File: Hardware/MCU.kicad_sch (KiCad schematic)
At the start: 37 parts, among them J5 Conn_01x05_Pin, Q1 BC847, SW1 SW_Push, SW2 SW_SPDT, U1 STM32F405RGT6, Y2 25MHz

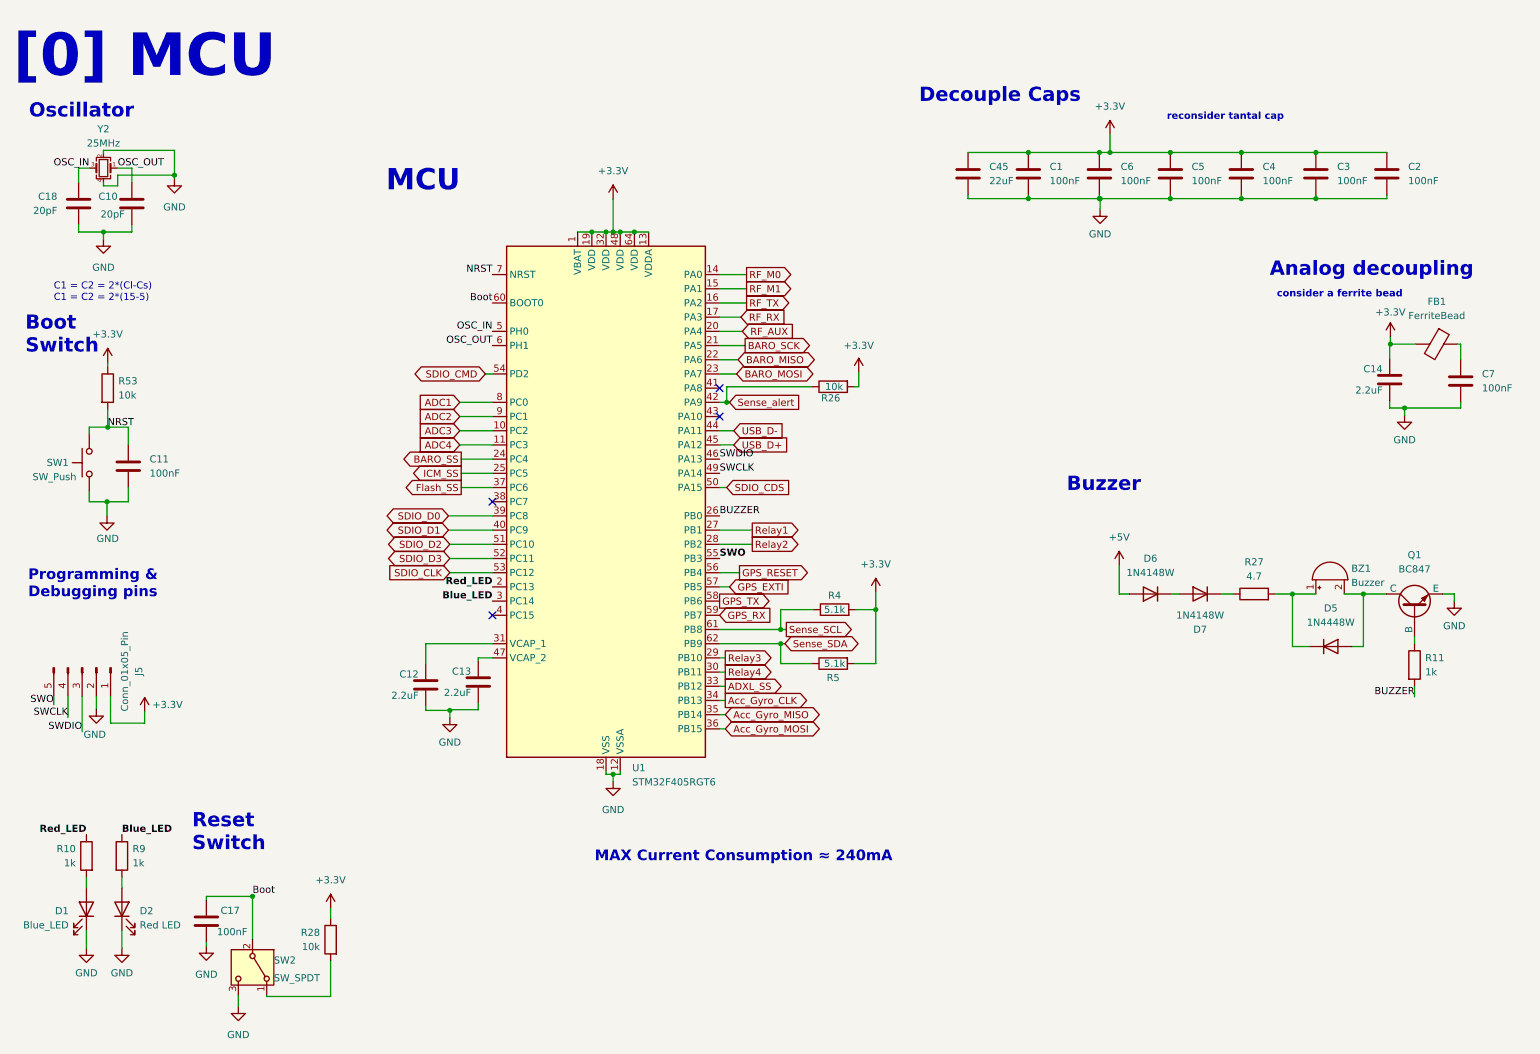
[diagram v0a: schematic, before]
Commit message: Changed footprints, generated BOM
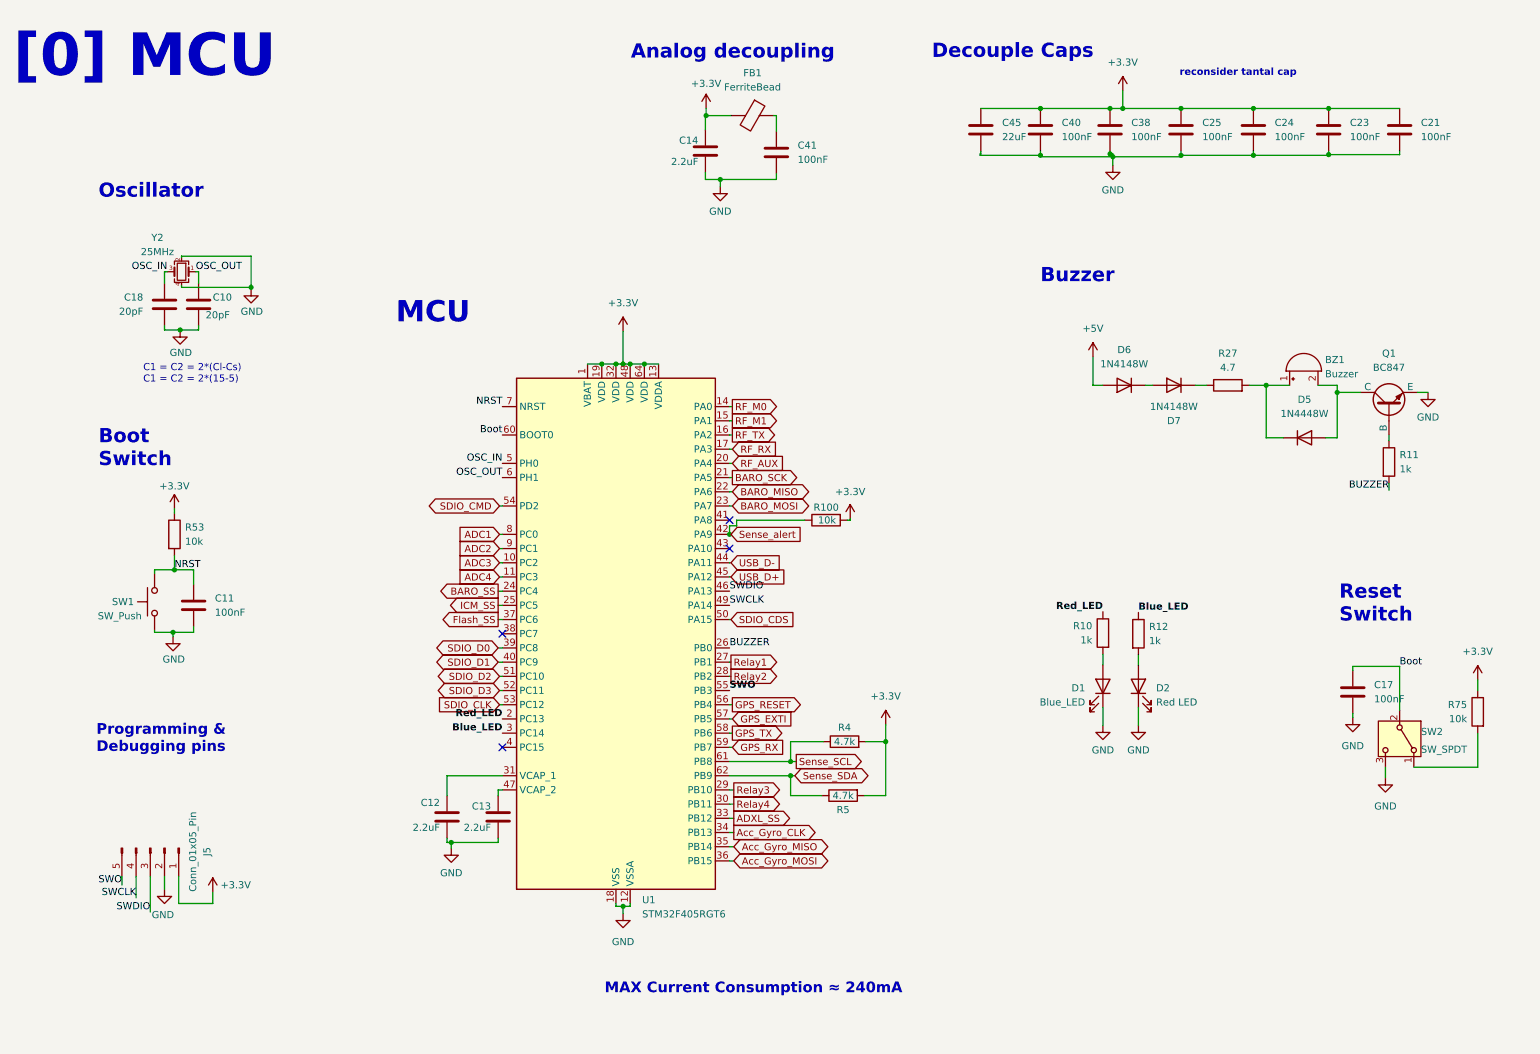
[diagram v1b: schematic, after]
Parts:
- removed C1, C2, C3, C4, C5, C6, C7: 100nF, Capacitor_SMD:C_0402_1005Metric, symbol Device:C
- removed R26, R28: 10k, Resistor_SMD:R_0402_1005Metric, symbol Device:R
- removed R9: 1k, Resistor_SMD:R_0402_1005Metric, symbol Device:R
- added C21, C23, C24, C25, C38, C40, C41: 100nF, Capacitor_SMD:C_0603_1608Metric, symbol Device:C
- added R100, R75: 10k, Resistor_SMD:R_0603_1608Metric, symbol Device:R
- added R12: 1k, Resistor_SMD:R_0603_1608Metric, symbol Device:R
- C11, C17: footprint Capacitor_SMD:C_0402_1005Metric -> Capacitor_SMD:C_0603_1608Metric; Distributer Link https://www.ozdisan.com/p/smt-smd-ve-mlcc-kapasitorler-184/murata-grt155r71e104ke01d-1074547 -> https://www.ozdisan.com/p/smt-smd-ve-mlcc-kapasitorler-184/samsung-cl10b104ko8wpnc-522227; Part Number GRT155R71E104KE01D -> CL10B104KO8WPNC
- R10, R11: footprint Resistor_SMD:R_0402_1005Metric -> Resistor_SMD:R_0603_1608Metric; Distributer Link https://www.ozdisan.com/p/smt-smd-ve-cip-direncler-194/roya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 -> https://www.ozdisan.com/p/smt-smd-ve-cip-direncler-194/vish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; Part Number HP02WAF1001TCE -> CRCW06031K00JNTABC
- R27: footprint Resistor_SMD:R_0402_1005Metric -> Resistor_SMD:R_0603_1608Metric; Distributer Link https://www.ozdisan.com/p/smt-smd-ve-cip-direncler-194/royalohm-cq02wgj047jtce-587859 -> https://www.ozdisan.com/p/smt-smd-ve-cip-direncler-194/royalohm-cq03saf470kt5e-587940; Part Number CQ02WGJ047JTCE -> CQ03SAF470KT5E
- R4, R5: value 5.1k -> 4.7k; footprint Resistor_SMD:R_0402_1005Metric -> Resistor_SMD:R_0603_1608Metric; Distributer Link https://www.ozdisan.com/p/smt-smd-ve-cip-direncler-194/pana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 -> https://www.ozdisan.com/p/smt-smd-ve-cip-direncler-194/roya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; Part Number ERJ2RKF5101X -> CQ03SAJ0472T5E
- R53: footprint Resistor_SMD:R_0402_1005Metric -> Resistor_SMD:R_0603_1608Metric; Distributer Link https://www.ozdisan.com/p/smt-smd-ve-cip-direncler-194/roya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 -> https://www.ozdisan.com/p/smt-smd-ve-cip-direncler-194/viki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; Part Number CQ02WGF1002TCE -> CRT03J7E1002
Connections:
- net +3.3V: now also C21.1, C23.1, C24.1, C25.1, C38.1, C40.1, R100.2, R75.1
- net Blue_LED: now also R12.1
- net GND: now also C21.2, C23.2, C24.2, C25.2, C38.2, C40.2, C41.2
- net NRST: now also C11.1, R53.2, SW1.2
- net Sense_alert: now also R100.1
- net at D2.2 (A): now also R12.2
- net at SW2.1 (A): now also R75.2
- net at FB1.1: now also C41.1
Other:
- note removed: "consider a ferrite bead"
- moved on the sheet: BZ1, C10, C11, C12, C13, C14, C18, C45, D1, D2, D5, D6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

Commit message: :)
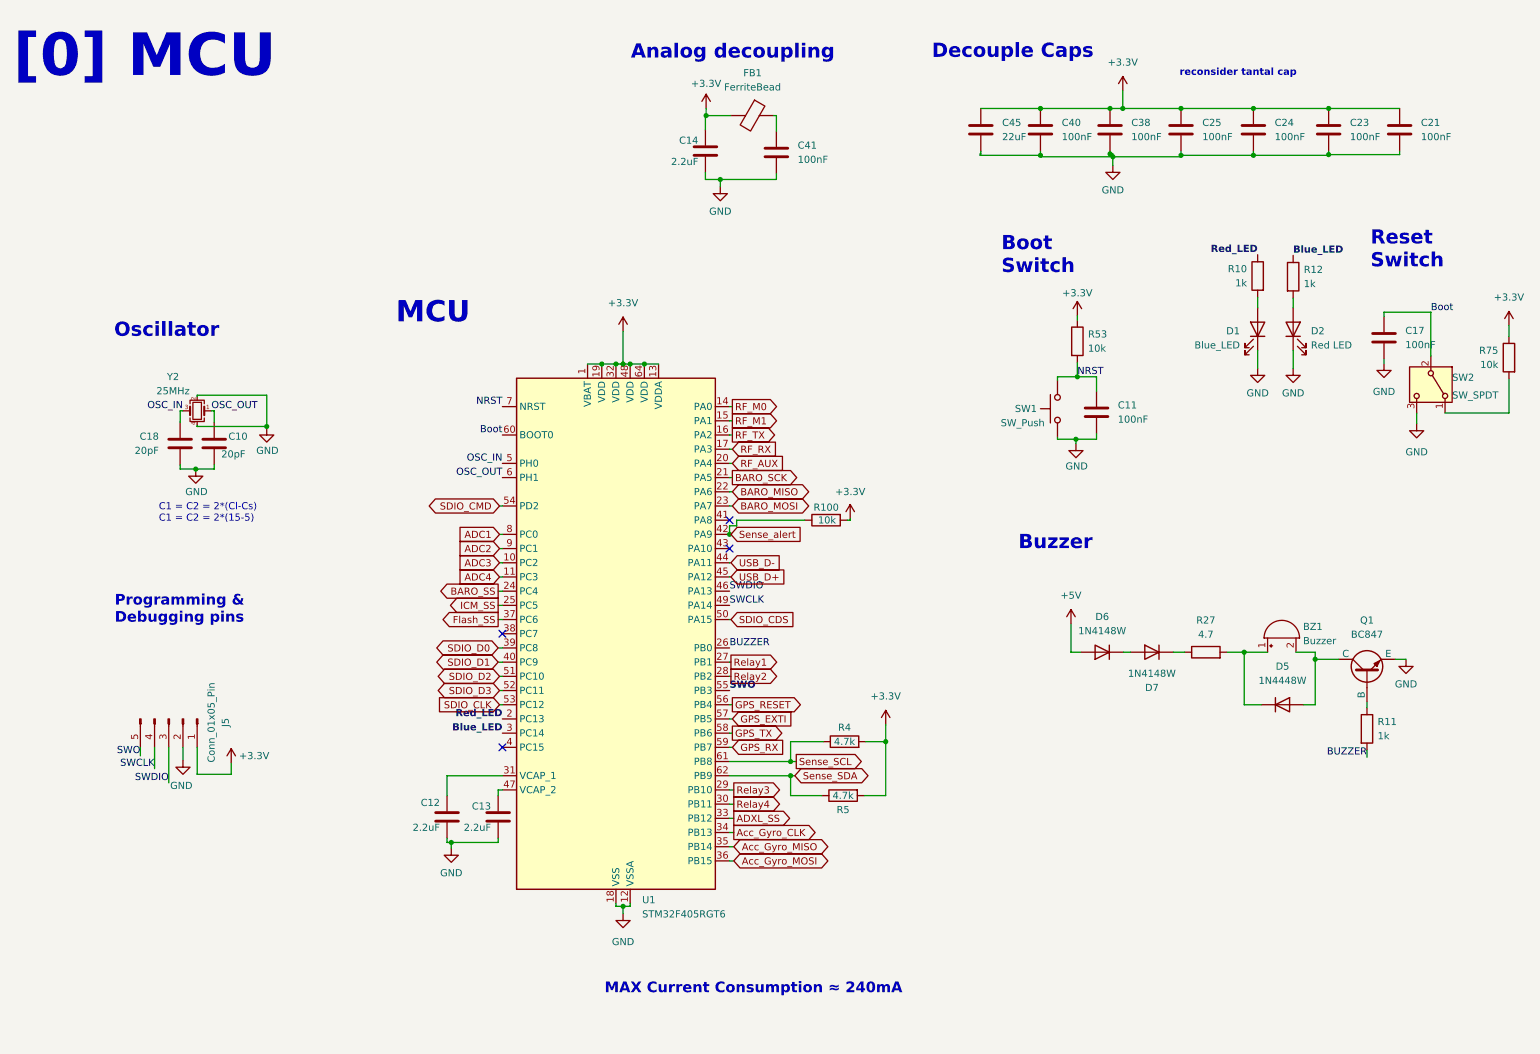
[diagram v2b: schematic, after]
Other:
- moved on the sheet: BZ1, C10, C11, C17, C18, D1, D2, D5, D6, D7, J5, Q1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
